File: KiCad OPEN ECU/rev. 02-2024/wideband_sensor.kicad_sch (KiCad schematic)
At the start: 21 parts, among them U12 CJ125

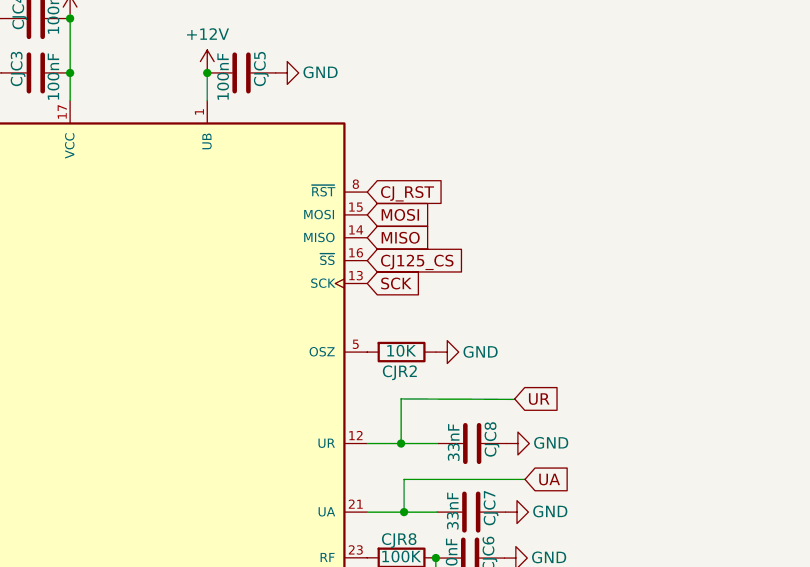
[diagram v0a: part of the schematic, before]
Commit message: update
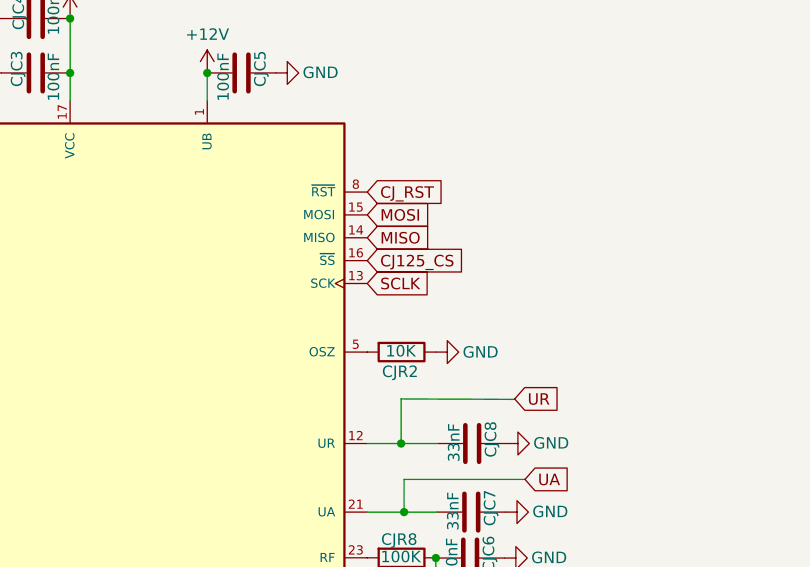
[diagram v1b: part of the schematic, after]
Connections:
- net SCK renamed SCLK
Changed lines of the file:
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@@
     )
   )
-  (global_label "SCK" (shape input) (at 171.5262 70.8406 0) (fields_autoplaced)
+  (global_label "SCLK" (shape input) (at 171.5262 70.8406 0) (fields_autoplaced)
     (effects (font (size 1.27 1.27)) (justify left))
-    (property "Intersheetrefs" "${INTERSHEET_REFS}" (at 177.6067 70.8406 0)
+    (property "Intersheetrefs" "${INTERSHEET_REFS}" (at 178.6348 70.8406 0)
       (effects (font (size 1.27 1.27)) (justify left) hide)
     )
